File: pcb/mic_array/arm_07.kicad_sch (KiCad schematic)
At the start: 16 parts, among them U57 IM72D128V01XTMA1, U58 IM72D128V01XTMA1, U59 IM72D128V01XTMA1, U60 IM72D128V01XTMA1, U61 IM72D128V01XTMA1, U62 IM72D128V01XTMA1, U63 IM72D128V01XTMA1, U64 IM72D128V01XTMA1

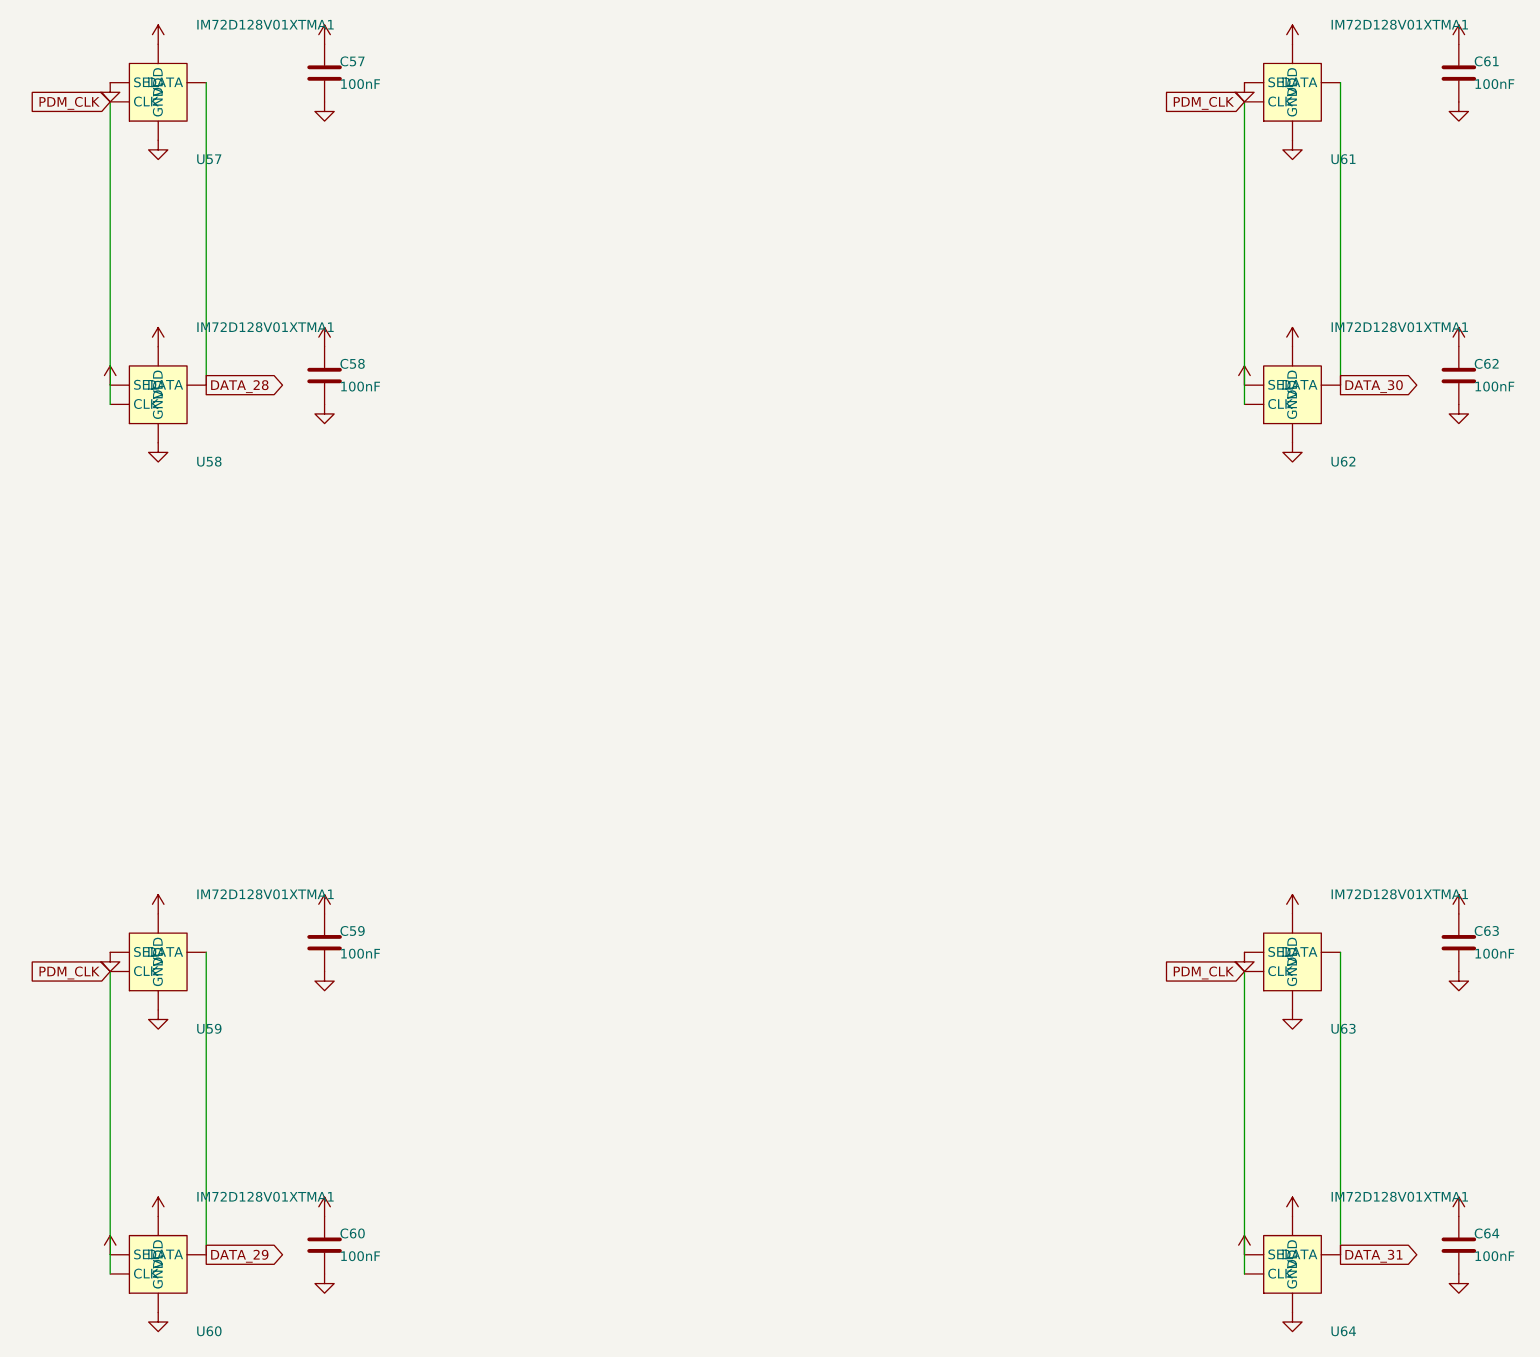
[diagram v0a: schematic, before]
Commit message: Updated.
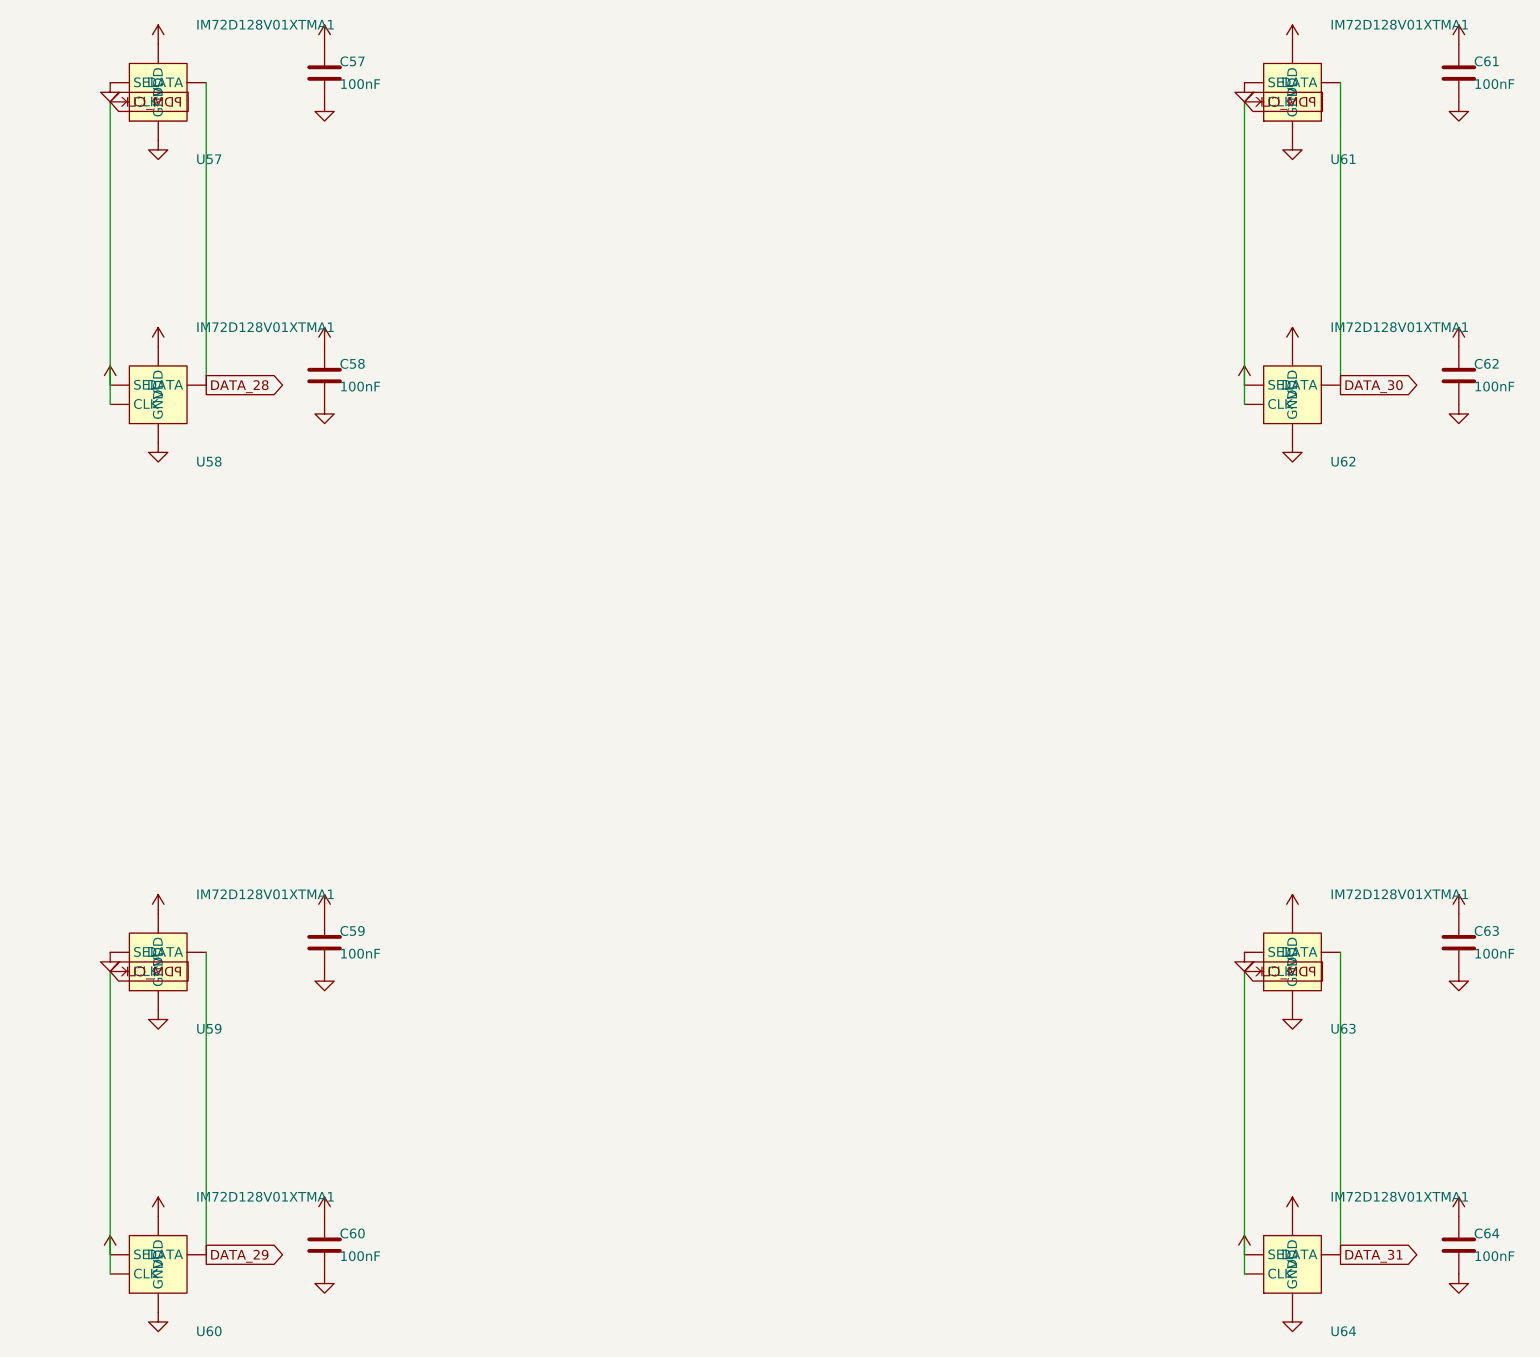
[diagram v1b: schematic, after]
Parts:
- C57, C58, C59, C60, C61, C62, C63, C64: footprint Capacitor_SMD:C_0402_1005Metric -> (none)
- U57, U58, U59, U60, U61, U62, U63, U64: footprint Sensor_Audio:Infineon_PG-LLGA-5-2 -> (none)
